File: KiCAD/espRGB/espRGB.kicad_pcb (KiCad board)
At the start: 2 copper layers, 56.5 x 39.4 mm, 16 parts, among them J1 Conn_01x04_Female, J2 Conn_01x02_Female, Q1 Q_PNP_BEC, Q2 Q_NPN_BEC, Q3 Q_PNP_BEC, Q4 Q_NPN_BEC, Q5 Q_PNP_BEC, Q6 Q_NPN_BEC, Q7 Q_NMOS_GSD, Q8 Q_NMOS_GSD, Q9 Q_NMOS_GSD, U1 WeMos_D1_mini

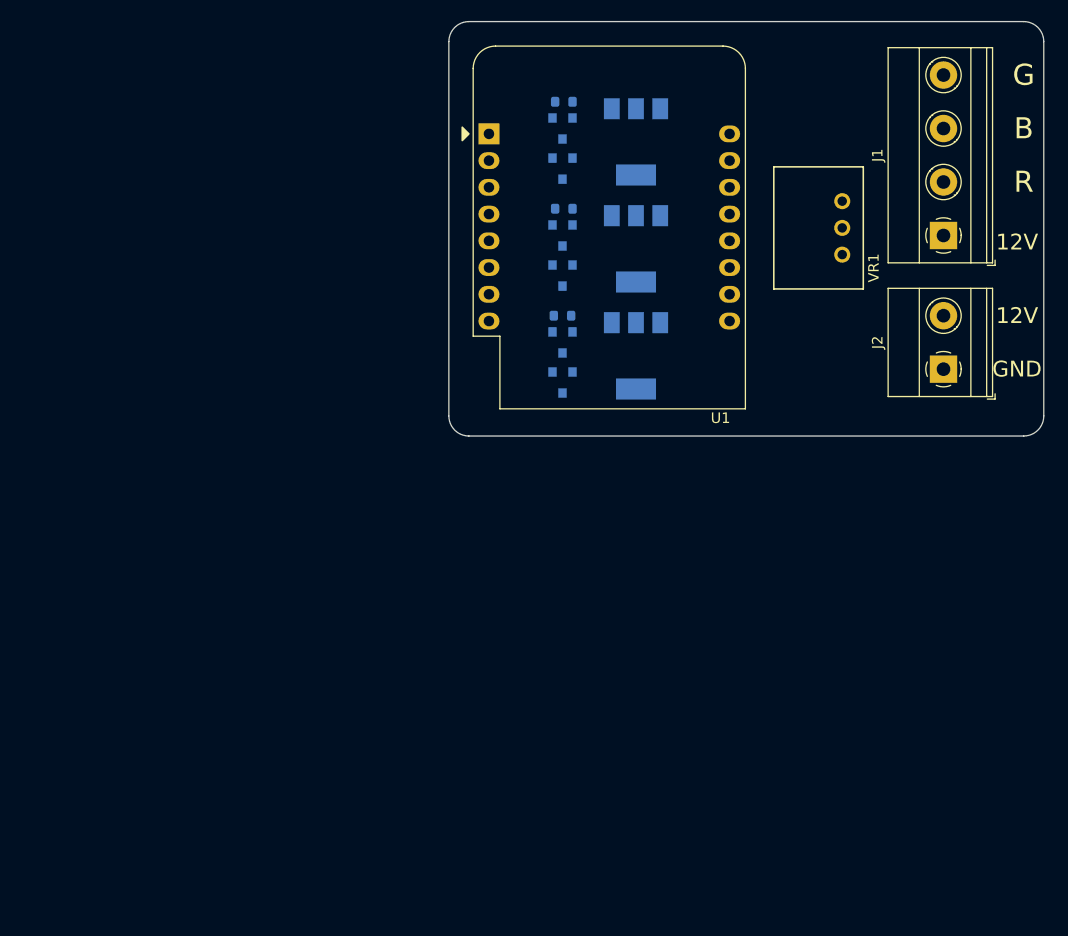
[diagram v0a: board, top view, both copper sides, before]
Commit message: v1.1
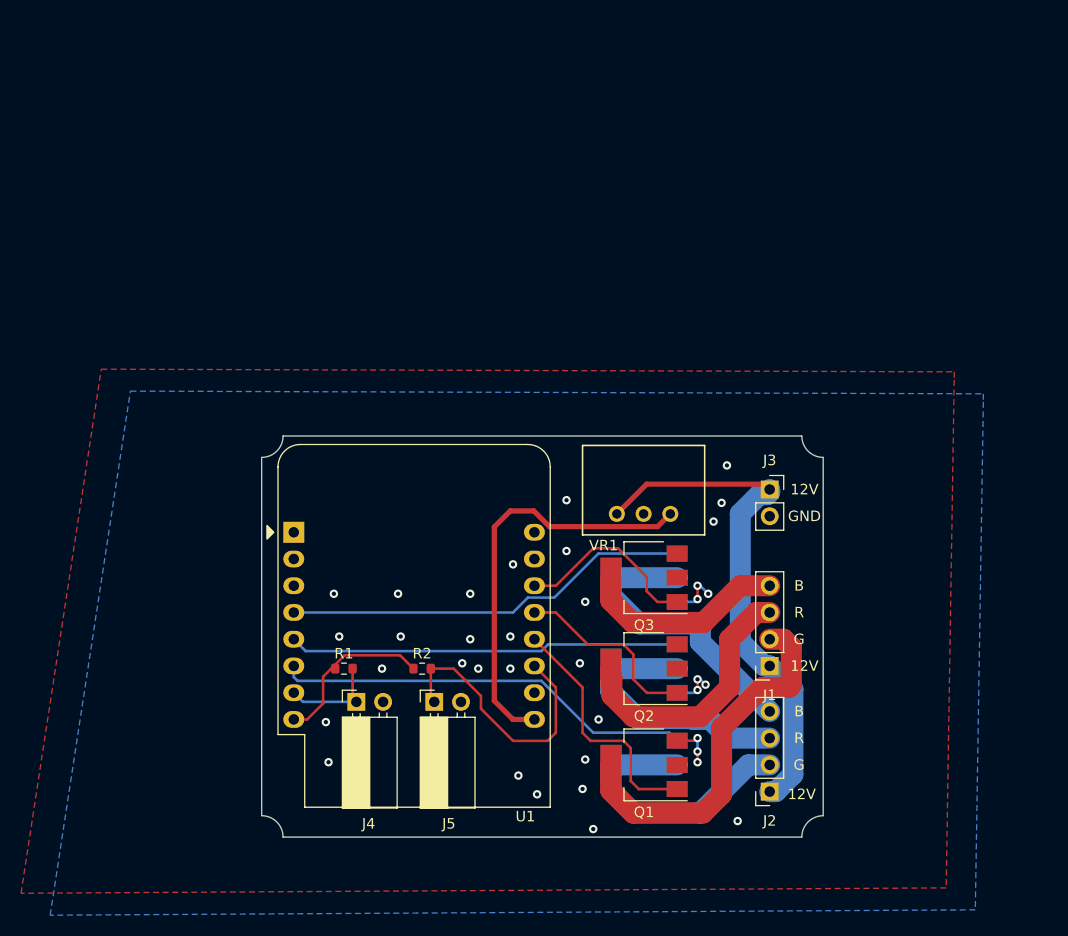
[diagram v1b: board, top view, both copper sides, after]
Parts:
- removed Q7, Q8, Q9: Q_NMOS_GSD, Package_TO_SOT_SMD:SOT-223-3_TabPin2
- removed R3: R, Resistor_SMD:R_0603_1608Metric
- added J3: Conn_01x02_Female, Connector_PinSocket_2.54mm:PinSocket_1x02_P2.54mm_Vertical, F.Cu at (123.2, 118.1)
- added J4: Conn_01x02_Female, Connector_PinSocket_2.54mm:PinSocket_1x02_P2.54mm_Horizontal, F.Cu at (83.9, 138.3)
- added J5: Conn_01x02_Female, Connector_PinSocket_2.54mm:PinSocket_1x02_P2.54mm_Horizontal, F.Cu at (91.3, 138.3)
- added REF**: OSHW-Logo2_9.8x8mm_SilkScreen, Symbol:OSHW-Logo2_9.8x8mm_SilkScreen, B.Cu at (87.9, 126.2)
- J1: footprint TerminalBlock_Phoenix:TerminalBlock_Phoenix_MKDS-1,5-4-5.08_1x04_P5.08mm_Horizontal -> Connector_PinSocket_2.54mm:PinSocket_1x04_P2.54mm_Vertical
- J2: value Conn_01x02_Female -> Conn_01x04_Female; footprint TerminalBlock_Phoenix:TerminalBlock_Phoenix_MKDS-1,5-2-5.08_1x02_P5.08mm_Horizontal -> Connector_PinSocket_2.54mm:PinSocket_1x04_P2.54mm_Vertical
- Q1, Q3: value Q_PNP_BEC -> Q_NMOS_GDS; footprint Package_TO_SOT_SMD:SOT-23 -> Package_TO_SOT_SMD:SOT-223-3_TabPin2; moved to F.Cu
- Q2: value Q_NPN_BEC -> Q_NMOS_GDS; footprint Package_TO_SOT_SMD:SOT-23 -> Package_TO_SOT_SMD:SOT-223-3_TabPin2; moved to F.Cu
- Q4, Q6: value Q_NPN_BEC -> Q_NMOS_GDS; footprint Package_TO_SOT_SMD:SOT-23 -> Package_TO_SOT_SMD:SOT-223-3_TabPin2
- Q5: value Q_PNP_BEC -> Q_NMOS_GDS; footprint Package_TO_SOT_SMD:SOT-23 -> Package_TO_SOT_SMD:SOT-223-3_TabPin2
- R1, R2: moved to F.Cu
- moved Q4 60.9 mm to (111.3, 144.3), turned to 180 degrees
- moved R2 55.5 mm to (90.2, 135.1), turned to 0 degrees
- moved R1 48.4 mm to (82.7, 135.1), turned to 0 degrees
- moved Q1 47.1 mm to (111.3, 144.3), turned to 180 degrees
- moved J1 44.1 mm to (123.2, 134.9), turned to 180 degrees
- moved J2 43.4 mm to (123.2, 146.8), turned to 180 degrees
- moved U1 42.1 mm to (78.0, 122.2)
- moved Q2 41.9 mm to (111.3, 135.1), turned to 180 degrees
- moved Q3 39.6 mm to (111.3, 126.5), turned to 180 degrees
- moved VR1 35.5 mm to (105.4, 122.4), turned to 0 degrees
- moved Q5 28.3 mm to (111.3, 135.1), turned to 180 degrees
- moved Q6 23.7 mm to (111.3, 126.5), turned to 180 degrees
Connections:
- J1 pad 2: /red_out -> /green2
- J1 pad 3: /blue_out -> /red2
- J1 pad 4: /green_out -> /blue2
- J2 pad 1: GND -> +12V
- J2 pad 2: +12V -> /green1
- Q1 pad 1: Net-(Q1-Pad1) -> /green2_gate
- Q1 pad 2: +5V -> /green2
- Q1 pad 3: Net-(Q1-Pad3) -> GND
- Q2 pad 1: Net-(Q1-Pad1) -> /red2_gate
- Q2 pad 2: GND -> /red2
- Q2 pad 3: Net-(Q1-Pad3) -> GND
- Q3 pad 1: Net-(Q3-Pad1) -> /blue2_gate
- Q3 pad 2: +5V -> /blue2
- Q3 pad 3: Net-(Q3-Pad3) -> GND
- Q4 pad 1: Net-(Q3-Pad1) -> /green1_gate
- Q4 pad 2: GND -> /green1
- Q4 pad 3: Net-(Q3-Pad3) -> GND
- Q5 pad 1: Net-(Q5-Pad1) -> /red1_gate
- Q5 pad 2: +5V -> /red1
- Q5 pad 3: Net-(Q5-Pad3) -> GND
- Q6 pad 1: Net-(Q5-Pad1) -> /blue1_gate
- Q6 pad 2: GND -> /blue1
- Q6 pad 3: Net-(Q5-Pad3) -> GND
- R1 pad 1: Net-(Q1-Pad1) -> +3V3
- R1 pad 2: /red -> /button1
- R2 pad 1: Net-(Q3-Pad1) -> +3V3
- R2 pad 2: /blue -> /button2
- U1 pad 11: /green -> /button2
- U1 pad 12: /red -> /green2_gate
- U1 pad 13: Net-(U1-Pad13) -> /red2_gate
- U1 pad 14: Net-(U1-Pad14) -> /blue2_gate
- U1 pad 3: /blue -> Net-(U1-Pad3)
- U1 pad 4: Net-(U1-Pad4) -> /blue1_gate
- U1 pad 5: Net-(U1-Pad5) -> /red1_gate
- U1 pad 6: Net-(U1-Pad6) -> /green1_gate
- U1 pad 7: Net-(U1-Pad7) -> /button1
- U1 pad 8: Net-(U1-Pad8) -> +3V3
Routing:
- net +12V: track 0.00 -> 49.8 mm
- net /green1_gate: track 0.00 -> 40.0 mm
- net +5V: track 0.00 -> 39.5 mm
- net /blue1_gate: track 0.00 -> 38.7 mm
- net /red1_gate: track 0.00 -> 37.2 mm
- net /green2: track 0.00 -> 35.2 mm
- net /blue1: track 0.00 -> 28.4 mm
- net /green1: track 0.00 -> 26.6 mm
- net /button2: track 0.00 -> 26.5 mm
- net /red1: track 0.00 -> 25.4 mm
- net /red2: track 0.00 -> 25.2 mm
- net /green2_gate: track 0.00 -> 23.8 mm
- net /blue2: track 0.00 -> 19.6 mm
- net /red2_gate: track 0.00 -> 18.1 mm
- net /blue2_gate: track 0.00 -> 17.9 mm
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- added copper zone on B.Cu, net GND
- added copper zone on F.Cu, net GND
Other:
- board size 56.5 x 39.4 mm -> 53.3 x 38.1 mm
- board text added: "espRGB - v1.1 github.com/jagjordi/espRGB"
